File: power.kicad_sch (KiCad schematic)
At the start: 71 parts, among them SW1 SW_Push, U3 BD71847MWV, Y1 32.768Khz

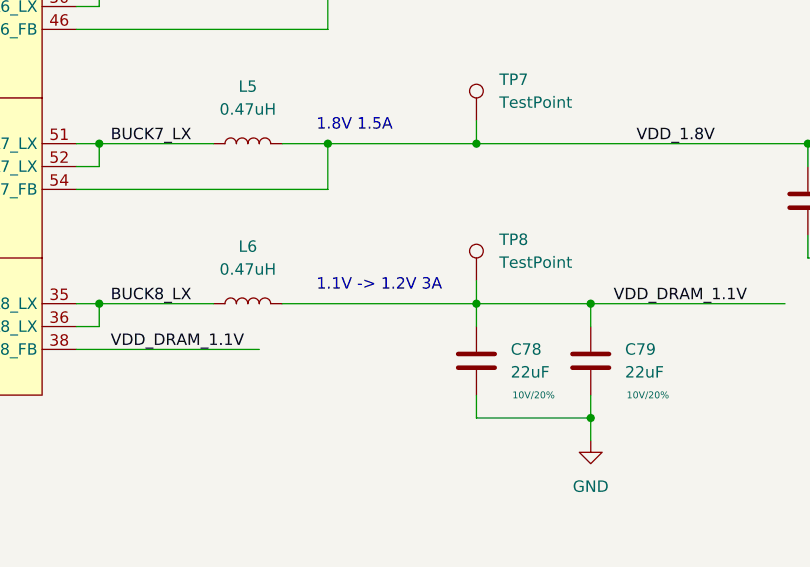
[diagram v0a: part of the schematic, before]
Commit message: Rev 1
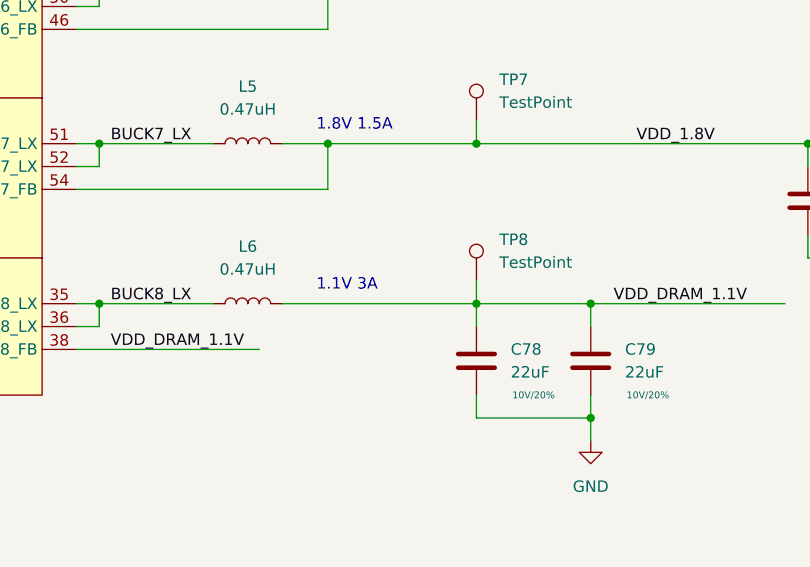
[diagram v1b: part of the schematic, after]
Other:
- note added: "1.1V 3A"
- note removed: "1.1V -> 1.2V 3A"
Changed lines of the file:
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@@
   (title_block
     (title "QSBC")
-    (rev "1")
+    (date "2022-12-01")
+    (rev "1.0")
     (company "Q-LAB")
   )
@@
     (effects (font (size 1.27 1.27)) (justify left bottom))
   )
-  (text "1.1V -> 1.2V 3A\n" (at 196.85 139.7 0)
+  (text "1.1V 3A\n" (at 196.85 139.7 0)
     (effects (font (size 1.27 1.27)) (justify left bottom))
   )
